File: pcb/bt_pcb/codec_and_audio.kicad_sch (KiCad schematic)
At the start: 20 parts, among them IC2 ADAU1961WBCPZ-R7, J3 Conn_01x01, J4 Conn_01x03

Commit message: made a bom
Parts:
- J3, J4: now left out of the parts list
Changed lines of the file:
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@@
 		(dnp no)
 		(fields_autoplaced yes)
-		(property "Reference" "#PWR027"
+		(property "Reference" "#PWR028"
 			(at 62.23 81.28 0)
 			(effects
@@
 			(project ""
 				(path "/eb787481-08cd-41a4-a128-173fa6227c32/4ada0139-8712-47ce-9d4c-ab8fef312f7b"
-					(reference "#PWR027")
+					(reference "#PWR028")
 					(unit 1)
 				)
@@
 			)
 		)
+		(property "Sim.Device" ""
+			(at 76.2 83.82 0)
+			(effects
+				(font
+					(size 1.27 1.27)
+				)
+				(hide yes)
+			)
+		)
 		(pin "1"
 		)
@@
 		(dnp no)
 		(fields_autoplaced yes)
-		(property "Reference" "#PWR025"
+		(property "Reference" "#PWR026"
 			(at 107.95 72.39 0)
 			(effects
@@
 			(project "bt_pcb"
 				(path "/eb787481-08cd-41a4-a128-173fa6227c32/4ada0139-8712-47ce-9d4c-ab8fef312f7b"
-					(reference "#PWR025")
+					(reference "#PWR026")
 					(unit 1)
 				)
@@
 			)
 		)
+		(property "Sim.Device" ""
+			(at 53.34 119.38 90)
+			(effects
+				(font
+					(size 1.27 1.27)
+				)
+				(hide yes)
+			)
+		)
 		(pin "1"
 		)
@@
 			)
 		)
+		(property "Sim.Device" ""
+			(at 143.51 156.21 90)
+			(effects
+				(font
+					(size 1.27 1.27)
+				)
+				(hide yes)
+			)
+		)
 		(pin "1"
 		)
@@
 		(dnp no)
 		(fields_autoplaced yes)
-		(property "Reference" "#PWR028"
+		(property "Reference" "#PWR029"
 			(at 189.23 92.71 0)
 			(effects
@@
 			(project "bt_pcb"
 				(path "/eb787481-08cd-41a4-a128-173fa6227c32/4ada0139-8712-47ce-9d4c-ab8fef312f7b"
-					(reference "#PWR028")
+					(reference "#PWR029")
 					(unit 1)
 				)
@@
 			)
 		)
+		(property "Sim.Device" ""
+			(at 62.23 83.82 0)
+			(effects
+				(font
+					(size 1.27 1.27)
+				)
+				(hide yes)
+			)
+		)
 		(pin "1"
 		)
@@
 		(dnp no)
 		(fields_autoplaced yes)
-		(property "Reference" "#PWR031"
+		(property "Reference" "#PWR032"
 			(at 110.49 139.7 0)
 			(effects
@@
 			(project "bt_pcb"
 				(path "/eb787481-08cd-41a4-a128-173fa6227c32/4ada0139-8712-47ce-9d4c-ab8fef312f7b"
-					(reference "#PWR031")
+					(reference "#PWR032")
 					(unit 1)
 				)
@@
 			)
 		)
+		(property "Sim.Device" ""
+			(at 93.98 96.52 90)
+			(effects
+				(font
+					(size 1.27 1.27)
+				)
+				(hide yes)
+			)
+		)
 		(pin "1"
 		)
@@
 		(dnp no)
 		(fields_autoplaced yes)
-		(property "Reference" "#PWR029"
+		(property "Reference" "#PWR030"
 			(at 62.23 93.98 0)
 			(effects
@@
 			(project "bt_pcb"
 				(path "/eb787481-08cd-41a4-a128-173fa6227c32/4ada0139-8712-47ce-9d4c-ab8fef312f7b"
-					(reference "#PWR029")
+					(reference "#PWR030")
 					(unit 1)
 				)
@@
 			)
 		)
+		(property "Sim.Device" ""
+			(at 87.63 36.83 0)
+			(effects
+				(font
+					(size 1.27 1.27)
+				)
+				(hide yes)
+			)
+		)
 		(pin "1"
 		)
@@
 			)
 		)
+		(property "Sim.Device" ""
+			(at 189.23 82.55 0)
+			(effects
+				(font
+					(size 1.27 1.27)
+				)
+				(hide yes)
+			)
+		)
 		(pin "1"
 		)
@@
 					(size 1.27 1.27)
 				)
+			)
+		)
+		(property "Sim.Device" ""
+			(at 76.2 139.7 0)
+			(effects
+				(font
+					(size 1.27 1.27)
+				)
+				(hide yes)
 			)
 		)
@@
 			)
 		)
+		(property "Sim.Device" ""
+			(at 62.23 36.83 0)
+			(effects
+				(font
+					(size 1.27 1.27)
+				)
+				(hide yes)
+			)
+		)
 		(pin "1"
 		)
@@
 		(dnp no)
 		(fields_autoplaced yes)
-		(property "Reference" "#PWR023"
+		(property "Reference" "#PWR024"
 			(at 74.93 34.29 0)
 			(effects
@@
 			(project ""
 				(path "/eb787481-08cd-41a4-a128-173fa6227c32/4ada0139-8712-47ce-9d4c-ab8fef312f7b"
-					(reference "#PWR023")
+					(reference "#PWR024")
 					(unit 1)
 				)
@@
 				)
 				(justify left top)
+				(hide yes)
+			)
+		)
+		(property "Sim.Device" ""
+			(at 101.6 93.98 0)
+			(effects
+				(font
+					(size 1.27 1.27)
+				)
 				(hide yes)
 			)
@@
 		(dnp no)
 		(fields_autoplaced yes)
-		(property "Reference" "#PWR032"
+		(property "Reference" "#PWR033"
 			(at 76.2 154.94 0)
 			(effects
@@
 			(project "bt_pcb"
 				(path "/eb787481-08cd-41a4-a128-173fa6227c32/4ada0139-8712-47ce-9d4c-ab8fef312f7b"
-					(reference "#PWR032")
+					(reference "#PWR033")
 					(unit 1)
 				)
@@
 		(unit 1)
 		(exclude_from_sim no)
-		(in_bom yes)
+		(in_bom no)
 		(on_board yes)
 		(dnp no)
@@
 			)
 		)
+		(property "Sim.Device" ""
+			(at 259.08 135.89 0)
+			(effects
+				(font
+					(size 1.27 1.27)
+				)
+				(hide yes)
+			)
+		)
 		(pin "1"
 		)
@@
 			)
 		)
+		(property "Sim.Device" ""
+			(at 151.13 156.21 90)
+			(effects
+				(font
+					(size 1.27 1.27)
+				)
+				(hide yes)
+			)
+		)
 		(pin "1"
 		)
@@
 			)
 		)
+		(property "Sim.Device" ""
+			(at 60.96 119.38 90)
+			(effects
+				(font
+					(size 1.27 1.27)
+				)
+				(hide yes)
+			)
+		)
 		(pin "1"
 		)
@@
 					(size 1.27 1.27)
 				)
+			)
+		)
+		(property "Sim.Device" ""
+			(at 88.9 139.7 0)
+			(effects
+				(font
+					(size 1.27 1.27)
+				)
+				(hide yes)
 			)
 		)
@@
 		(dnp no)
 		(fields_autoplaced yes)
-		(property "Reference" "#PWR024"
+		(property "Reference" "#PWR025"
 			(at 74.93 52.07 0)
 			(effects
@@
 			(project "bt_pcb"
 				(path "/eb787481-08cd-41a4-a128-173fa6227c32/4ada0139-8712-47ce-9d4c-ab8fef312f7b"
-					(reference "#PWR024")
+					(reference "#PWR025")
 					(unit 1)
 				)
@@
 			)
 		)
+		(property "Sim.Device" ""
+			(at 100.33 36.83 0)
+			(effects
+				(font
+					(size 1.27 1.27)
+				)
+				(hide yes)
+			)
+		)
 		(pin "1"
 		)
@@
 			)
 		)
+		(property "Sim.Device" ""
+			(at 74.93 36.83 0)
+			(effects
+				(font
+					(size 1.27 1.27)
+				)
+				(hide yes)
+			)
+		)
 		(pin "1"
 		)
@@
 		(unit 1)
 		(exclude_from_sim no)
-		(in_bom yes)
+		(in_bom no)
 		(on_board yes)
 		(dnp no)
@@
 		)
 		(property "Description" "Generic connector, single row, 01x01, script generated (kicad-library-utils/schlib/autogen/connector/)"
+			(at 66.04 104.14 0)
+			(effects
+				(font
+					(size 1.27 1.27)
+				)
+				(hide yes)
+			)
+		)
+		(property "Sim.Device" ""
 			(at 66.04 104.14 0)
 			(effects
@@
 			)
 		)
+		(property "Sim.Device" ""
+			(at 36.83 36.83 0)
+			(effects
+				(font
+					(size 1.27 1.27)
+				)
+				(hide yes)
+			)
+		)
 		(pin "1"
 		)
@@
 					(size 1.27 1.27)
 				)
+			)
+		)
+		(property "Sim.Device" ""
+			(at 173.99 82.55 0)
+			(effects
+				(font
+					(size 1.27 1.27)
+				)
+				(hide yes)
 			)
 		)
@@
 		(dnp no)
 		(fields_autoplaced yes)
-		(property "Reference" "#PWR026"
+		(property "Reference" "#PWR027"
 			(at 142.24 72.39 0)
 			(effects
@@
 			(project "bt_pcb"
 				(path "/eb787481-08cd-41a4-a128-173fa6227c32/4ada0139-8712-47ce-9d4c-ab8fef312f7b"
-					(reference "#PWR026")
+					(reference "#PWR027")
 					(unit 1)
 				)
@@
 			)
 		)
+		(property "Sim.Device" ""
+			(at 49.53 36.83 0)
+			(effects
+				(font
+					(size 1.27 1.27)
+				)
+				(hide yes)
+			)
+		)
 		(pin "1"
 		)
@@
 		(dnp no)
 		(fields_autoplaced yes)
-		(property "Reference" "#PWR030"
+		(property "Reference" "#PWR031"
 			(at 173.99 105.41 0)
 			(effects
@@
 			(project "bt_pcb"
 				(path "/eb787481-08cd-41a4-a128-173fa6227c32/4ada0139-8712-47ce-9d4c-ab8fef312f7b"
-					(reference "#PWR030")
-					(unit 1)
-				)
+					(reference "#PWR031")
+					(unit 1)
+				)

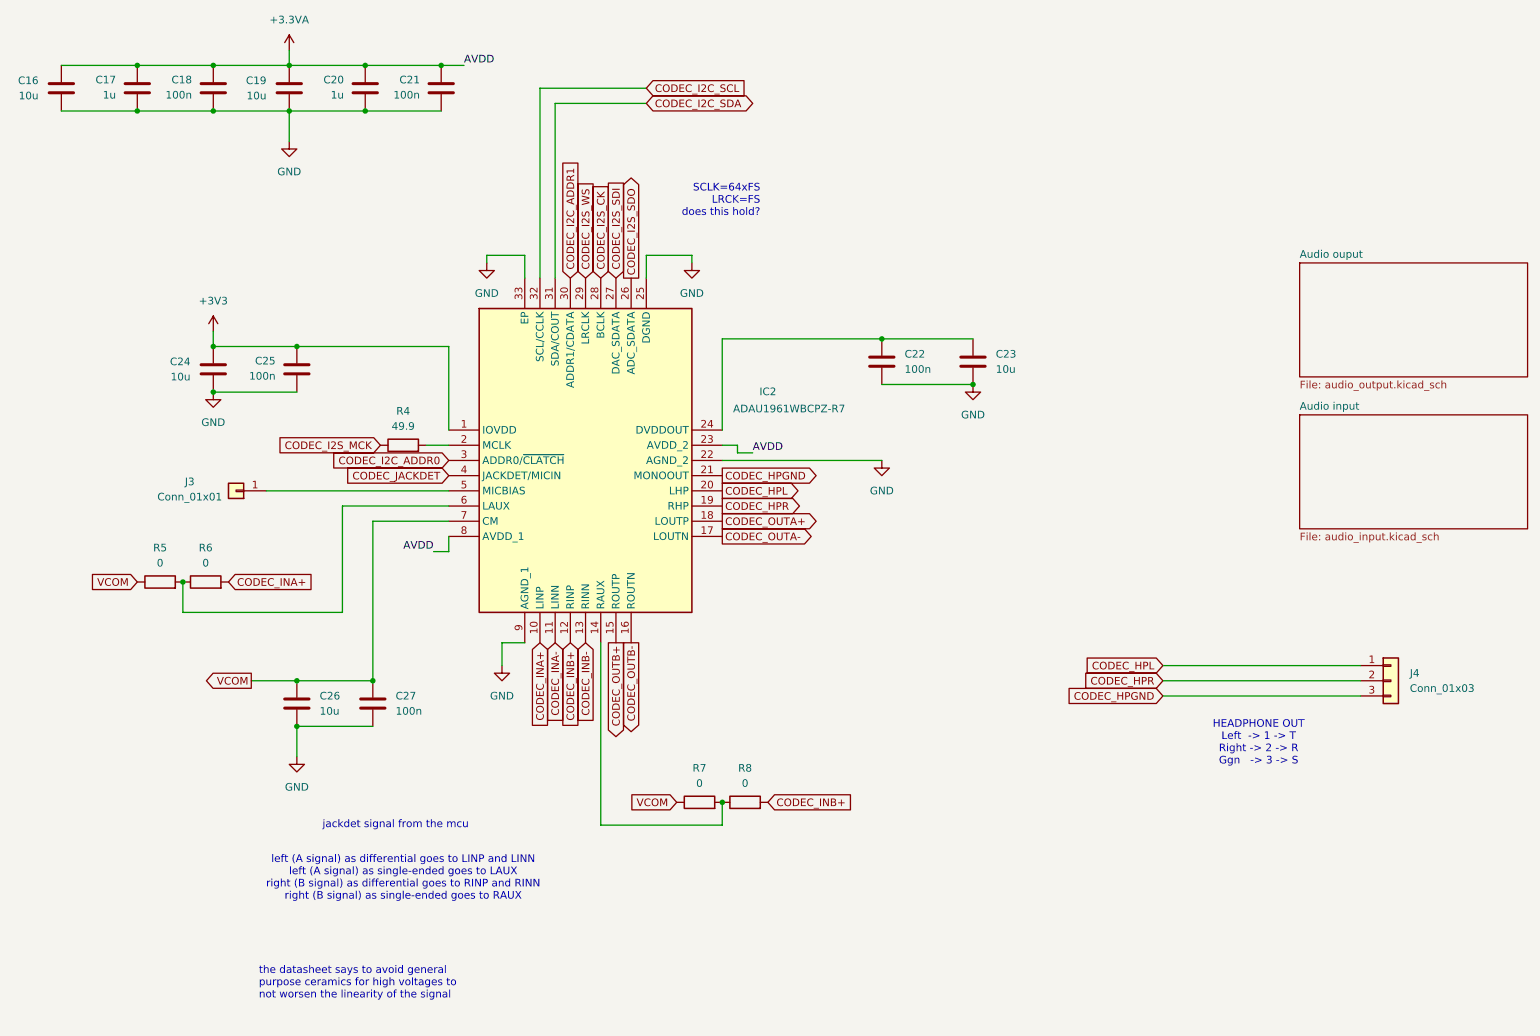
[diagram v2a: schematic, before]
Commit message: aaaaaaa
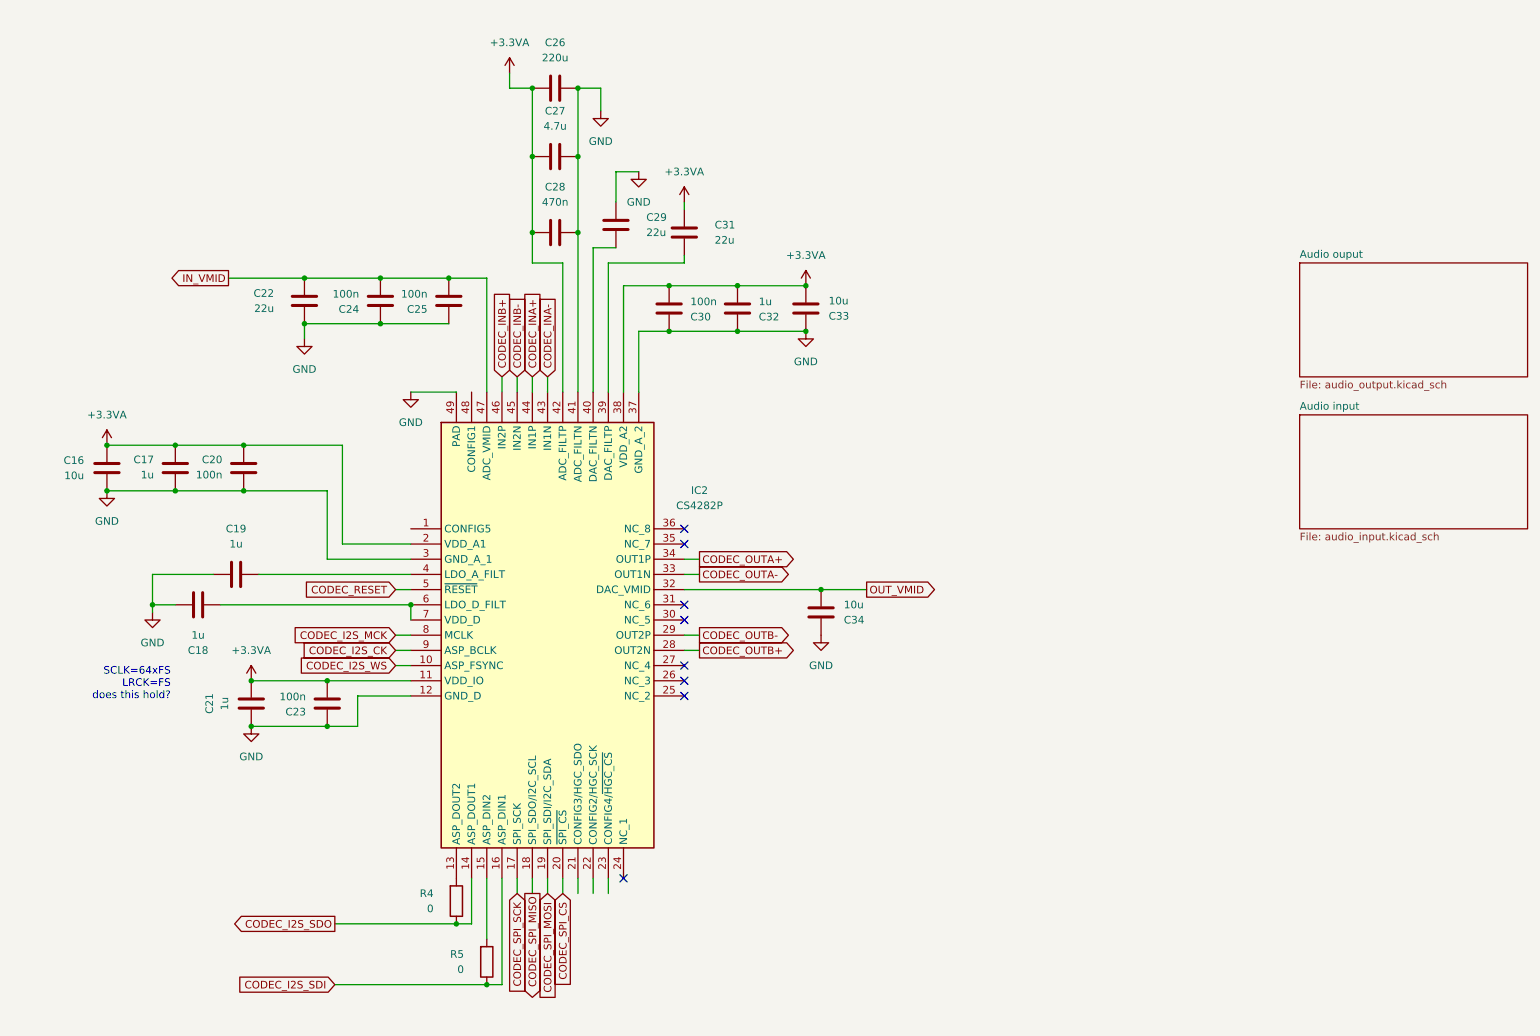
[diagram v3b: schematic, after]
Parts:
- removed C16: 10u, Capacitor_SMD:C_0805_2012Metric_Pad1.18x1.45mm_HandSolder, symbol Device:C
- removed C17: 1u, Capacitor_SMD:C_0603_1608Metric_Pad1.08x0.95mm_HandSolder, symbol Device:C
- removed IC2: ADAU1961WBCPZ-R7, library:QFN50P500X500X100-33N-D, symbol library:ADAU1961WBCPZ-R7
- removed J3: Conn_01x01, Connector_PinHeader_2.54mm:PinHeader_1x01_P2.54mm_Vertical, symbol Connector_Generic:Conn_01x01
- removed J4: Conn_01x03, Connector_JST:JST_PH_B3B-PH-K_1x03_P2.00mm_Vertical, symbol Connector_Generic:Conn_01x03
- removed R6, R7, R8: 0, Resistor_SMD:R_0603_1608Metric_Pad0.98x0.95mm_HandSolder, symbol Device:R
- added C19, C21, C32: 1u, Capacitor_SMD:C_0603_1608Metric_Pad1.08x0.95mm_HandSolder, symbol Device:C
- added C28: 470n, Capacitor_SMD:C_0603_1608Metric_Pad1.08x0.95mm_HandSolder, symbol Device:C
- added C29, C31: 22u, Capacitor_SMD:C_0805_2012Metric_Pad1.18x1.45mm_HandSolder, symbol Device:C
- added C30: 100n, Capacitor_SMD:C_0603_1608Metric_Pad1.08x0.95mm_HandSolder, symbol Device:C
- added C33, C34: 10u, Capacitor_SMD:C_0805_2012Metric_Pad1.18x1.45mm_HandSolder, symbol Device:C
- added IC2: CS4282P, library:QFN40P600X600X80-49N-D, symbol library:CS4282P
- C18: value 100n -> 1u
- C22: value 100n -> 22u; footprint Capacitor_SMD:C_0603_1608Metric_Pad1.08x0.95mm_HandSolder -> Capacitor_SMD:C_0805_2012Metric_Pad1.18x1.45mm_HandSolder
- C23, C24: value 10u -> 100n; footprint Capacitor_SMD:C_0805_2012Metric_Pad1.18x1.45mm_HandSolder -> Capacitor_SMD:C_0603_1608Metric_Pad1.08x0.95mm_HandSolder
- C26: value 10u -> 220u
- C27: value 100n -> 4.7u; footprint Capacitor_SMD:C_0603_1608Metric_Pad1.08x0.95mm_HandSolder -> Capacitor_SMD:C_0805_2012Metric_Pad1.18x1.45mm_HandSolder
- R4: value 49.9 -> 0
- renumbered C19 to C16, C20 to C17, C21 to C20
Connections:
- net +3V3 is gone; now on net GND: C24.1, C25.1
- net +3.3VA: now also C23.2, C26.1, C27.1, C21.1, C28.1, C30.2, C31.1, C32.2, C33.2, IC2.11 (VDD_IO), IC2.2 (VDD_A1), IC2.38 (VDD_A2), IC2.42 (ADC_FILTP); no longer C18.1
- net CODEC_I2S_CK: now also IC2.9 (ASP_BCLK)
- net CODEC_I2S_MCK: now also IC2.8 (MCLK); no longer R4.1
- net CODEC_I2S_SDI: now also R5.1, IC2.16 (ASP_DIN1)
- net CODEC_I2S_SDO: now also R4.1, IC2.14 (ASP_DOUT1)
- net CODEC_I2S_WS: now also IC2.10 (ASP_FSYNC)
- net CODEC_INA+: now also IC2.44 (IN1P)
- net CODEC_INA-: now also IC2.43 (IN1N)
- net CODEC_INB+: now also IC2.46 (IN2P)
- net CODEC_INB-: now also IC2.45 (IN2N)
- net CODEC_OUTA+: now also IC2.34 (OUT1P)
- net CODEC_OUTA-: now also IC2.33 (OUT1N)
- net CODEC_OUTB+: now also IC2.28 (OUT2N)
- net CODEC_OUTB-: now also IC2.29 (OUT2P)
- net GND: now also C23.1, C19.2, C21.2, C28.2, C29.1, C30.1, C32.1, C33.1, C34.1, IC2.12 (GND_D), IC2.3 (GND_A_1), IC2.37 (GND_A_2), IC2.41 (ADC_FILTN), IC2.49 (PAD); no longer C23.2, C24.2, C25.2
- net at R5.2: now also IC2.15 (ASP_DIN2)
- net at R4.2: now also IC2.13 (ASP_DOUT2)
- net IN_VMID: now reaches C22.1
- net IN_VMID: now also C24.2, C25.2, IC2.47 (ADC_VMID); no longer C23.1
- removed net VCOM: C26.1, C27.1, R5.1
- new net: C29.2, IC2.40 (DAC_FILTN)
- new net: C18.1, IC2.6 (LDO_D_FILT), IC2.7 (VDD_D)
- new net: C31.2, IC2.39 (DAC_FILTP)
- new net: C19.1, IC2.4 (LDO_A_FILT)
- new net CODEC_RESET: IC2.5 (~{RESET})
- new net CODEC_SPI_CS: IC2.20 (~{SPI_CS})
- new net CODEC_SPI_MISO: IC2.18 (SPI_SDO/I2C_SCL)
- new net CODEC_SPI_MOSI: IC2.19 (SPI_SDI/I2C_SDA)
- new net CODEC_SPI_SCK: IC2.17 (SPI_SCK)
- new net OUT_VMID: C34.2, IC2.32 (DAC_VMID)
- no-connect marks 0 -> 8
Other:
- note removed: "HEADPHONE OUT Left -> 1 -> T Right -> 2 -> R Ggn -> 3 -> S"
- note removed: "jackdet signal from the mcu"
- note removed: "left (A signal) as differential goes to LINP and LINN left (A signal) as single-ended goes to LAUX right (B signal) as differential goes to RINP and RINN right (B signal) as single-ended goes to RAUX"
- note removed: "the datasheet says to avoid general purpose ceramics for high voltages to not worsen the linearity of the signal"
- moved on the sheet: C16, C17, C20
